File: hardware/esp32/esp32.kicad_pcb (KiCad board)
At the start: 4 copper layers, 50 x 50 mm, 63 parts, among them J1 Screw_Terminal_01x02, J2 ESP_left, J3 ESP_right, Q1 MMBT5401, Q2 MMBT2222A, U2 LMV321, U3 LMV321, U4 mini_esp32, U5 HT7533-1, U6 LM393

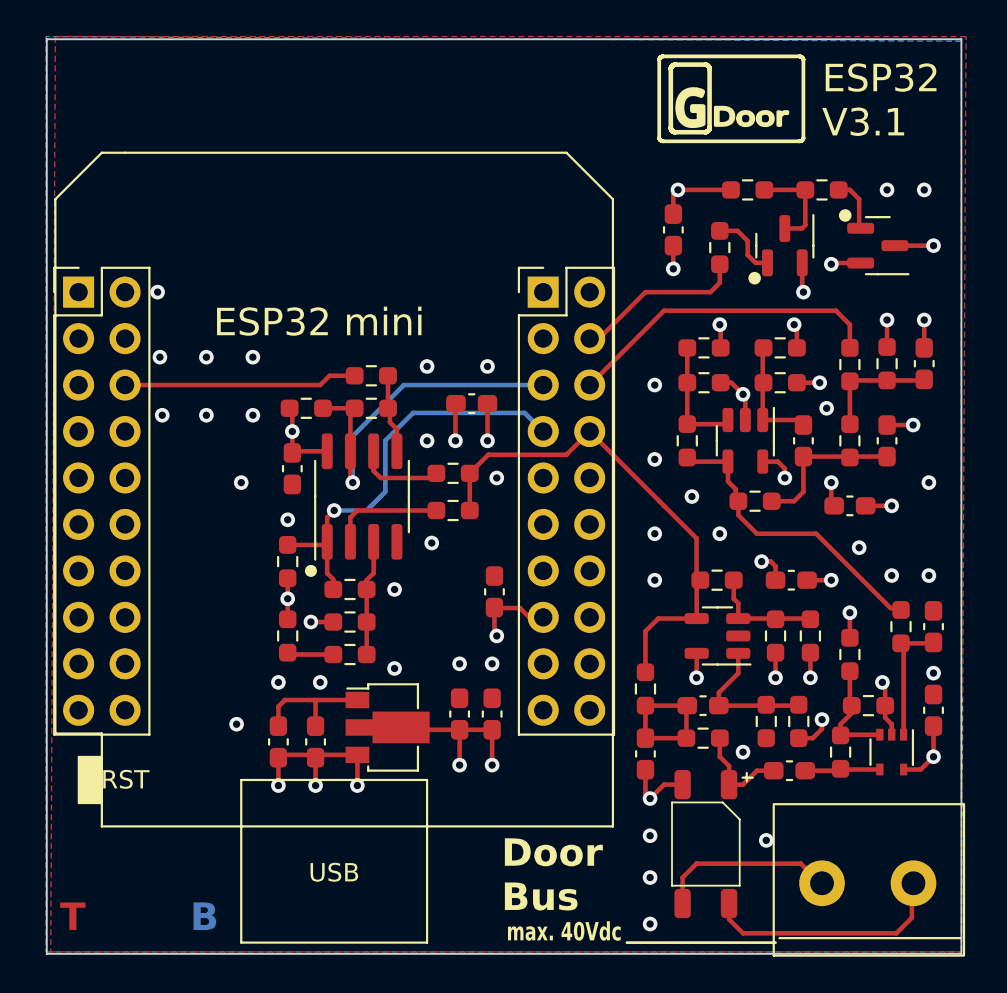
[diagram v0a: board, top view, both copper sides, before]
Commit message: Work on V3.1
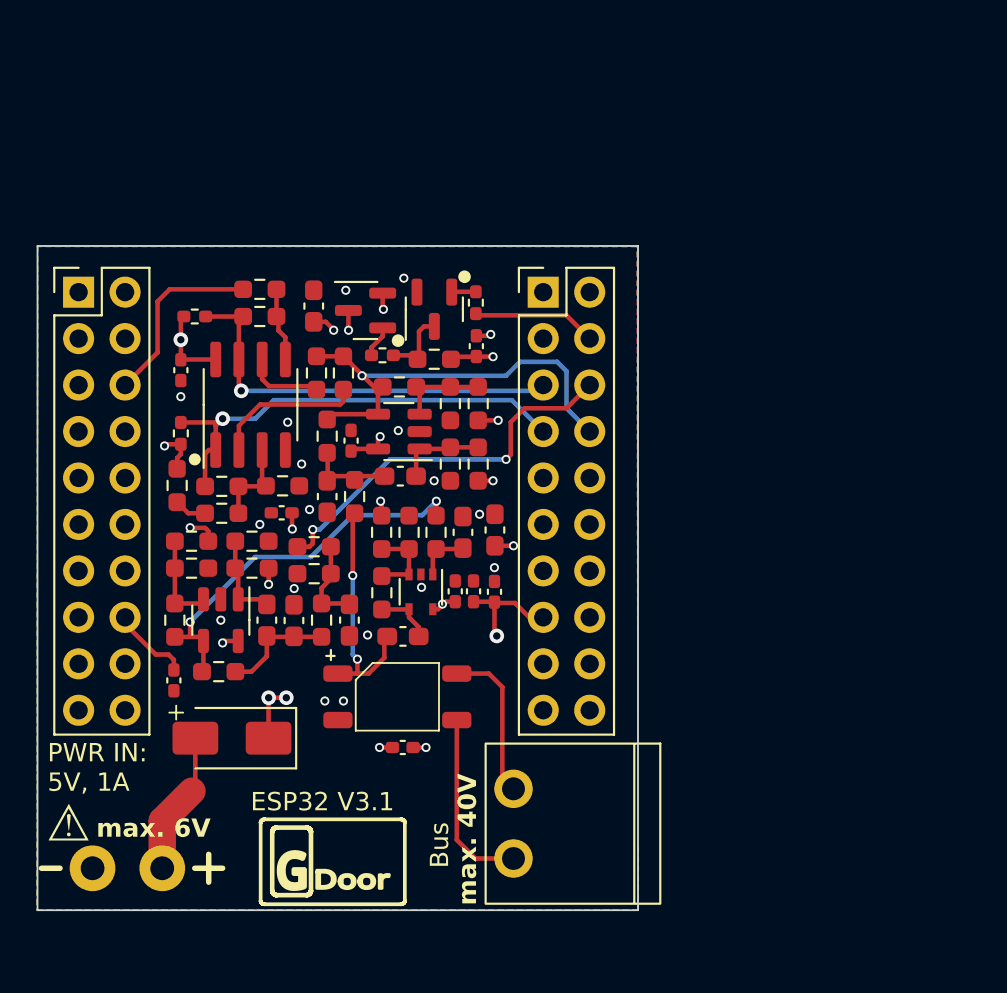
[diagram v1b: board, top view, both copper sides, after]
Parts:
- removed U5: HT7533-1, Library:SOT-89-3
- added D2: SS14, Library:D_SMA, F.Cu at (122.7, 104.6)
- added J4: PlugIn_Terminal_01x02, Library:steckklemme2x1_dnp, F.Cu at (117.0, 111.8)
- added J5: Plugged into C8387, Library:nofoorprint, F.Cu at (153.5, 109.4)
- added S1: SYM_ESD_Small, Library:ESD-Logo_6.6x6mm_SilkScreen, B.Cu at (123.4, 89.5)
- C11, C13, C15, C16, C17, C5, C6, C7: footprint Library:C_0603_1608Metric_Pad1.08x0.95mm_HandSolder -> Library:C_0402_1005Metric_Pad0.74x0.62mm_HandSolder
- C3: value 10n -> 100n; footprint Library:C_0603_1608Metric_Pad1.08x0.95mm_HandSolder -> Library:C_0402_1005Metric_Pad0.74x0.62mm_HandSolder
- J1: value Screw_Terminal_01x02 -> PlugIn_Terminal_01x02; footprint Library:anschlussklemme2x1 -> Library:steckklemme2x1_1
- R13, R29, R31, R8: footprint Library:R_0603_1608Metric_Pad0.98x0.95mm_HandSolder -> Library:R_0402_1005Metric_Pad0.72x0.64mm_HandSolder
- U4: value mini_esp32 -> ~
- moved C10 34.4 mm to (129.1, 98.2), turned to 90 degrees
- moved C9 33.9 mm to (126.1, 98.2)
- moved R21 33.4 mm to (127.2, 95.7), turned to 0 degrees
- moved C7 31.1 mm to (125.4, 92.3), turned to 180 degrees
- moved R34 30.9 mm to (127.2, 94.2), turned to 180 degrees
- moved C8 30.9 mm to (124.6, 98.2)
- moved R15 30.8 mm to (122.0, 101.0)
- moved R19 30.8 mm to (123.8, 93.9)
- moved R18 30.6 mm to (123.8, 95.4)
- moved R20 30.5 mm to (127.6, 98.2)
- moved U3 30.3 mm to (122.1, 98.2)
- moved R17 29.9 mm to (120.5, 93.9)
- moved R16 29.8 mm to (120.5, 95.4)
- moved R14 29.7 mm to (119.6, 98.2)
- moved Q1 28.2 mm to (130.0, 81.3), turned to 0 degrees
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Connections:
- D1 pad 3: Net-(J1-Pin_1) -> Net-(J1-Pin_2)
- D1 pad 4: Net-(J1-Pin_2) -> Net-(J1-Pin_1)
- J2 pad 16: unconnected-(J2-3V3-Pad16) -> +3.3V
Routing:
- net GND: track 32.8 -> 2.02 mm, vias 54 -> 19
- net +5V: track 26.6 -> 13.5 mm, vias 5 -> 6
- net Net-(D2-A): track 0.00 -> 7.86 mm
- net Net-(D1-+): track 5.51 -> 13.0 mm, vias 0 -> 2
- net +3.3V: track 24.2 -> 17.3 mm, vias 10 -> 7
- net /5V_onoff: track 12.8 -> 7.66 mm
- net Net-(R11-Pad1): track 16.8 -> 21.2 mm, vias 0 -> 2
- net /TX: track 17.4 -> 21.1 mm, vias 0 -> 2
- net Net-(U1-+): track 6.59 -> 2.96 mm
- net Net-(C2-Pad2): track 8.10 -> 4.68 mm
- net Net-(J1-Pin_2): track 13.4 -> 10.1 mm
- net /RX_ANA: track 27.7 -> 24.4 mm, vias 0 -> 1
- net /RX: track 22.3 -> 25.3 mm
- net Net-(U2-+): track 7.69 -> 4.80 mm
- net /RX_DAC: track 20.1 -> 22.6 mm
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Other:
- board size 50 x 50 mm -> 32.8 x 36.3 mm
- board text added: "5V PWR in"
- board text added: "A"
- board text added: "Bus"
- board text added: "ESP 3.3Vout"
- board text added: "ESP 5Vout"
- board text added: "ESP32Mini"
- board text added: "PWR IN: 5V, 1A"
- board text added: "github.com/ gdoor-org/gdoor"
- board text added: "max. 40V"
- board text added: "max. 6V"
- board text added: "⚠"
- board text removed: "*) Debug Pins"
- board text removed: "5Vin"
- board text removed: "5Vin: max. 6V, 100mA"
- board text removed: "Analog in: RX_THRESH* (0-3.3V)"
- board text removed: "Analog out: RX_ANA* (0-3.3V)"
- board text removed: "Bus A"
- board text removed: "Bus B"
- board text removed: "Door Bus"
- board text removed: "ESP32 mini"
- board text removed: "GPIO in: TX, TX_EN"
- board text removed: "GPIO out: RX, RX_DAC*"
- board text removed: "I1"
- board text removed: "I2"
- board text removed: "T"
- board text removed: "https://github.com/gdoor-org/gdoor"
- board text removed: "max. 40Vdc"
